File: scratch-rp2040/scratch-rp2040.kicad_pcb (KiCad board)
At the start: 2 copper layers, 32 parts, among them P1 USB_C_Plug_USB2.0, SW1 SW_SPST, SW2 SW_SPST, SW3 SW_SPST, SW4 SW_SPST, SW5 SW_SPST, SW6 SW_SPST, SW7 SW_SPST, U1 RP2040, U2 NCP1117-3.3_SOT223, U3 W25Q128JVS, Y1 12MHz

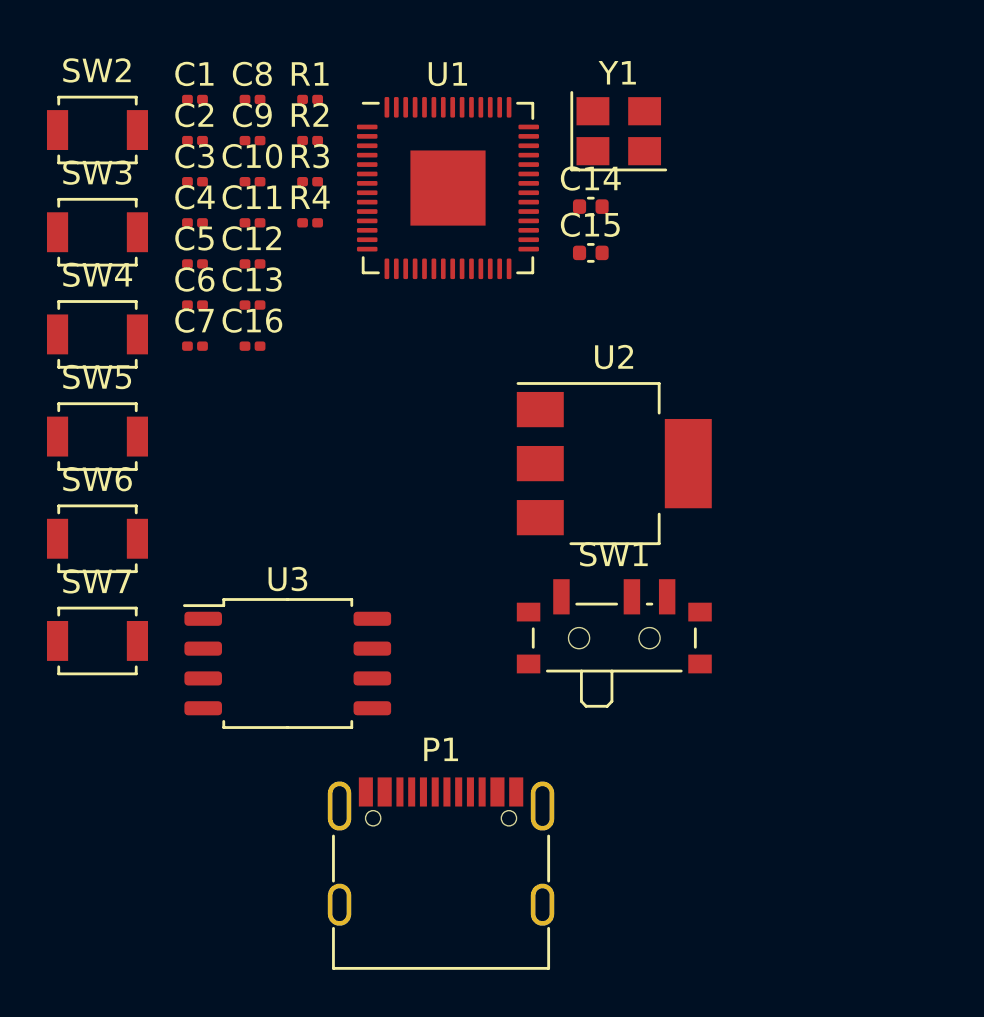
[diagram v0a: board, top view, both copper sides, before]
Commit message: parts placed
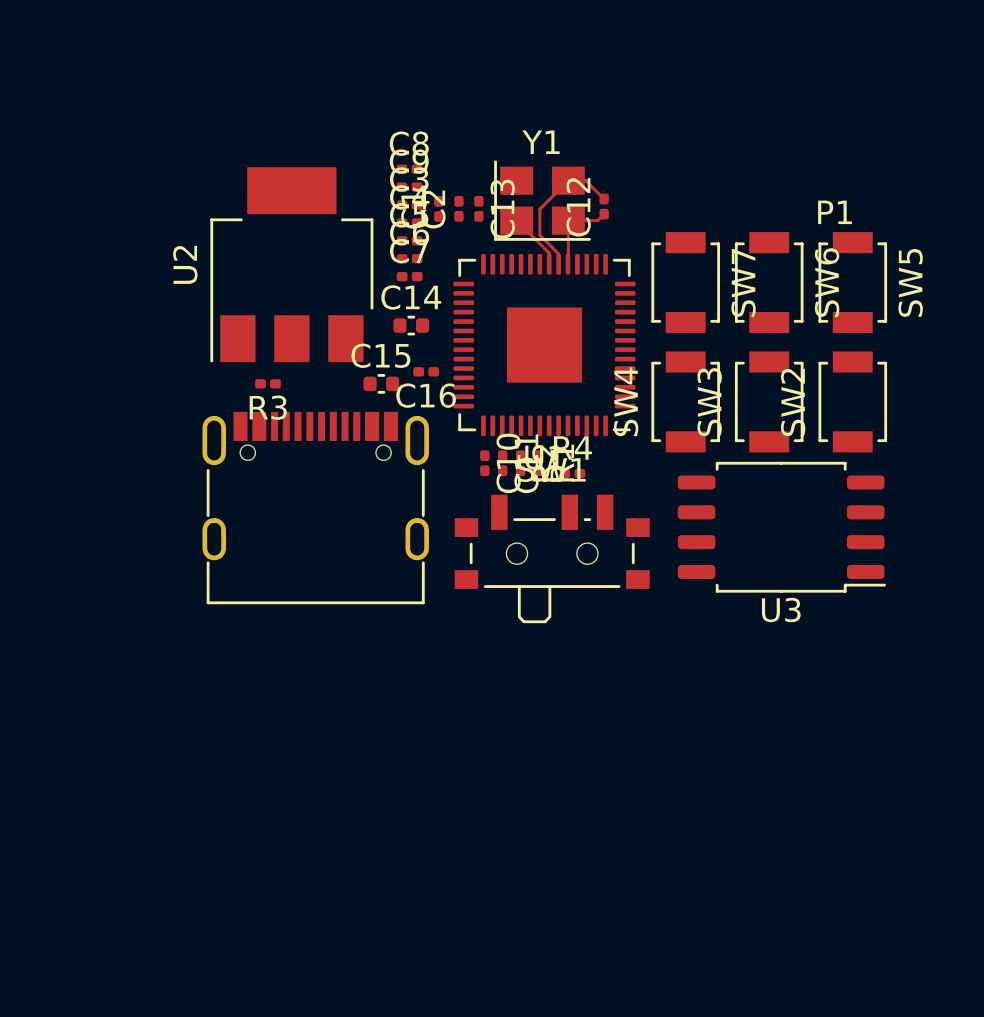
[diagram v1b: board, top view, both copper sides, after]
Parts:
- moved SW2 34.2 mm to (81.0, 42.7), turned to 90 degrees
- moved SW5 32.8 mm to (81.0, 37.6), turned to -90 degrees
- moved SW6 30.6 mm to (77.5, 37.6), turned to -90 degrees
- moved SW3 29.5 mm to (77.5, 42.7), turned to 90 degrees
- moved SW7 29.3 mm to (73.9, 37.6), turned to -90 degrees
- moved SW4 25.2 mm to (73.9, 42.7), turned to 90 degrees
- moved U3 21.8 mm to (78.0, 48.0), turned to 180 degrees
- moved R1 18.3 mm to (67.6, 45.3), turned to -90 degrees
- moved P1 16.5 mm to (58.2, 47.4)
- moved R2 16.4 mm to (66.9, 45.3), turned to -90 degrees
- moved U2 16.1 mm to (57.1, 36.8), turned to 90 degrees
- moved C10 15.5 mm to (65.4, 45.3), turned to -90 degrees
- moved R4 15.4 mm to (69.1, 45.7)
- moved C12 15.2 mm to (70.4, 34.4), turned to 90 degrees
- moved C11 14.8 mm to (66.1, 45.3), turned to -90 degrees
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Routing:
- net Net-(U1-XIN): track 0.00 -> 6.24 mm
- net GND: track 0.00 -> 4.00 mm
- net Net-(U1-XOUT): track 0.00 -> 2.43 mm
